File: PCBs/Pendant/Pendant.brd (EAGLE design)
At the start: 30.5 x 34.3 mm, 20 parts

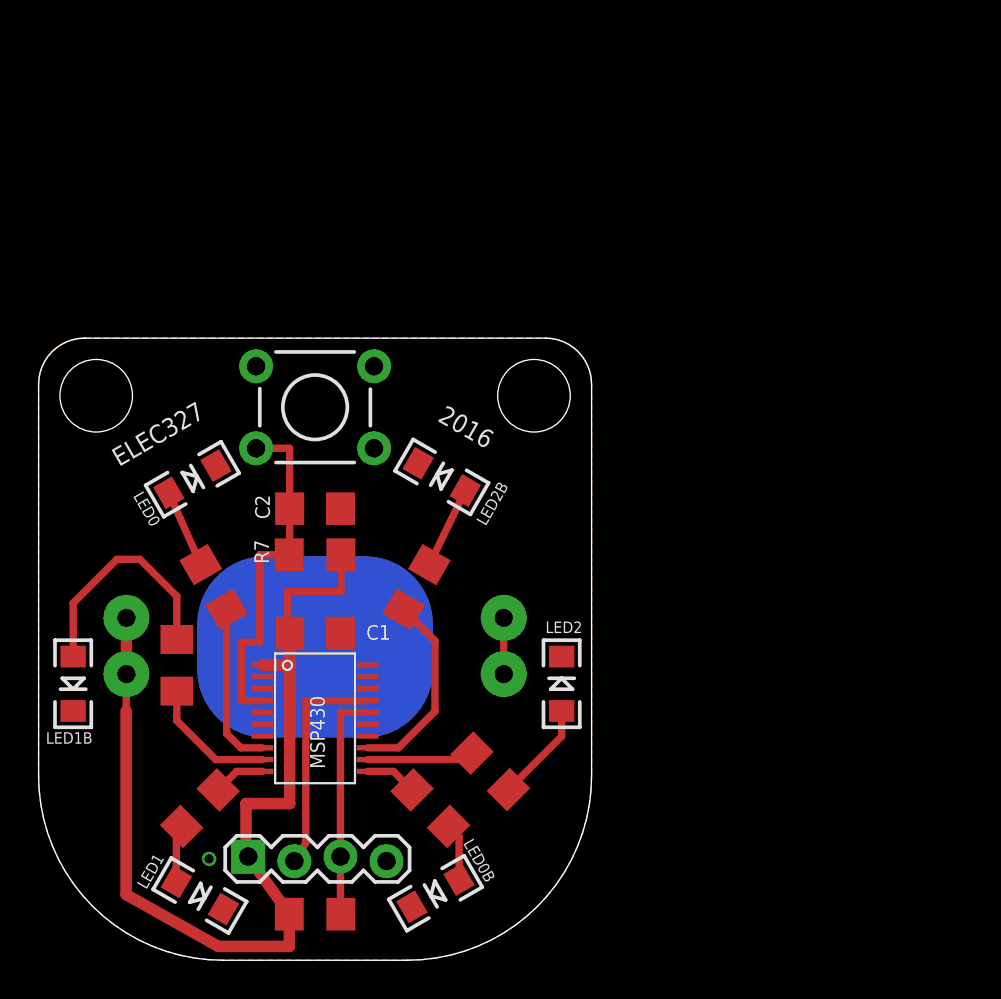
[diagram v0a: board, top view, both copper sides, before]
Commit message: Updated Pendant Eagle files
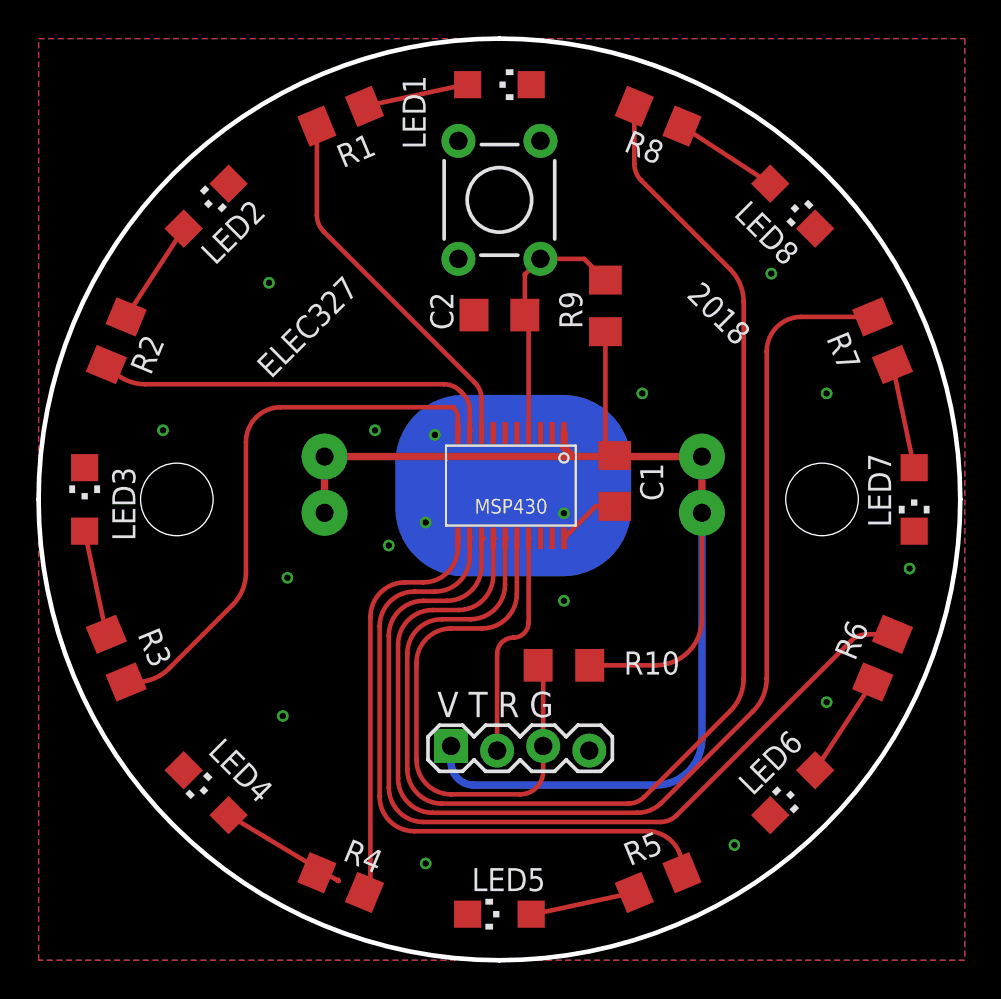
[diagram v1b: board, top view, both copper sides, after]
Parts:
- removed LED0, LED0B, LED1B, LED2B: (no value), SparkFun-LED:LED-1206
- removed R_PULLUP_RST: 43k, rcl:R1206
- added LED3, LED4, LED5, LED6, LED7, LED8: (no value), led:CHIPLED_1206
- added R10, R8, R9: (no value), rcl:R1206
- LED1, LED2: device SparkFun-LED:LED-1206 -> led:CHIPLED_1206
- moved LED1 47.6 mm to (25.4, 48.3), turned to 270 degrees
- moved R7 33.4 mm to (46.5, 34.1), turned to 292.5 degrees
- moved LED2 32.8 mm to (9.24, 41.6), turned to 315 degrees
- moved R1 26.9 mm to (16.7, 46.5), turned to 22.5 degrees
- moved R6 26.0 mm to (46.5, 16.7), turned to 247.5 degrees
- moved C1 18.5 mm to (31.8, 26.4), turned to 270 degrees
- moved R2 18.2 mm to (4.28, 34.1), turned to 67.5 degrees
- moved MSP430 16.8 mm to (26.0, 26.2), turned to 180 degrees
- moved S1 15.3 mm to (25.4, 41.9), turned to 90 degrees
- moved C2 14.7 mm to (25.4, 35.6), turned to 0 degrees
- moved BAT1 14.1 mm to (26.2, 26.2)
- moved JP1 12.7 mm to (22.7, 11.7)
- moved R5 11.1 mm to (34.1, 4.28), turned to 202.5 degrees
- moved R3 9.47 mm to (4.28, 16.7), turned to 112.5 degrees
- moved R4 6.42 mm to (16.7, 4.28), turned to 157.5 degrees
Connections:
- net N$1 renamed D5
- net N$2 renamed D4
- net N$5 renamed D6
- removed net N$10: LED1.A, R3.1
- removed net N$11: MSP430.8, R1.2
- removed net N$12: MSP430.9, R2.2
- removed net N$13: MSP430.10, R3.2
- removed net N$9: LED2B.A, R6.2
- new net D1: MSP430.8, R1.1
- new net D2: MSP430.9, R2.1
- new net D3: MSP430.10, R3.1
- new net D7: MSP430.14, R7.1
- new net D8: MSP430.15, R8.1
- new net N$1: LED1.A, R1.2
- new net N$2: LED2.A, R2.2
- new net N$5: LED5.A, R5.2
- net GND: now also LED3.C, LED4.C, LED5.C, LED6.C, LED7.C, LED8.C; no longer LED0.C, LED0B.C, LED1B.C, LED2B.C
- net N$14: now also R9.2; no longer R7.1
- net N$3: now also LED3.A, R3.2; no longer LED2.A, R5.2
- net N$4: now also LED4.A; no longer LED0B.A
- net N$6: now also LED6.A, R6.2; no longer MSP430.7
- net N$7: now also LED7.A, R7.2; no longer LED0.A, R1.1
- net N$8: now also LED8.A, R8.2; no longer LED1B.A, R2.1
- net VDD: now also R10.1, R9.1; no longer R7.2, R_PULLUP_RST.2
- net _RST: now also R10.2; no longer R_PULLUP_RST.1
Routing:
- net D8: track 0.00 -> 72.6 mm
- net D7: track 0.00 -> 66.0 mm
- net D6: track 10.9 -> 49.7 mm
- net D3: track 0.00 -> 30.6 mm
- net D5: track 5.90 -> 36.0 mm
- net D2: track 0.00 -> 22.6 mm
- net VDD: track 57.4 -> 79.8 mm
- net D1: track 0.00 -> 20.9 mm
- net D4: track 2.87 -> 22.9 mm
- net _RST: track 12.6 -> 29.8 mm
- net N$11: track 9.15 -> 0.00 mm
- net N$12: track 7.24 -> 0.00 mm
- net N$8: track 12.9 -> 6.08 mm
- net N$1: track 0.00 -> 6.19 mm
- net N$5: track 0.00 -> 6.14 mm
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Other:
- board size 30.5 x 34.3 mm -> 50.8 x 50.8 mm
- board text added: "2018"
- board text removed: "2016"
